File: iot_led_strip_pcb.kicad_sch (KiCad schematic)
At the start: 38 parts, among them J1 I2C Expansion, J2 Conn_01x03_Socket, J3 GT-USB-7010ASV, J4 Barrel_Jack_Switch_Pin3Ring, J5 TC2050-IDC_Cortex-M, J6 Conn_01x03_Socket_Solderwire, Q1 BSS138, SW1 RESET, SW2 FLASH, U2 ESP32-S2-MINI-1, Y1 Crystal_40Mhz

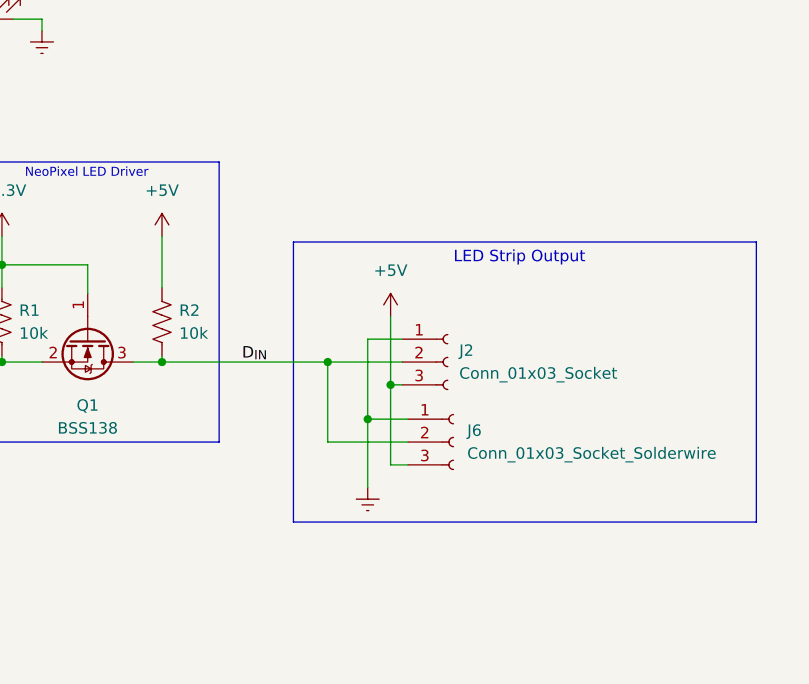
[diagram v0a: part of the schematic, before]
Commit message: final modifications, cleanup, added v2.0 photos as ordered
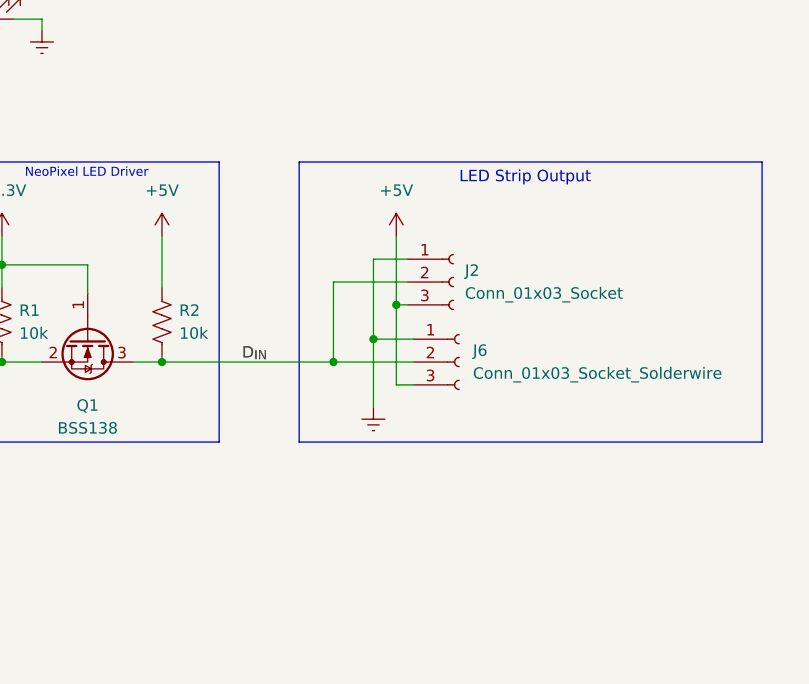
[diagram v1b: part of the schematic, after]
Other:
- title: Spotify Reactive IoT LED Strip Driver -> Spotify Neopixel Visualizer
- moved on the sheet: J2, J6
